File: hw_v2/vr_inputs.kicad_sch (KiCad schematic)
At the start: 26 parts, among them U1 MAX9924UAUB_, U7 74LVC2G17, U9 74LVC2G17

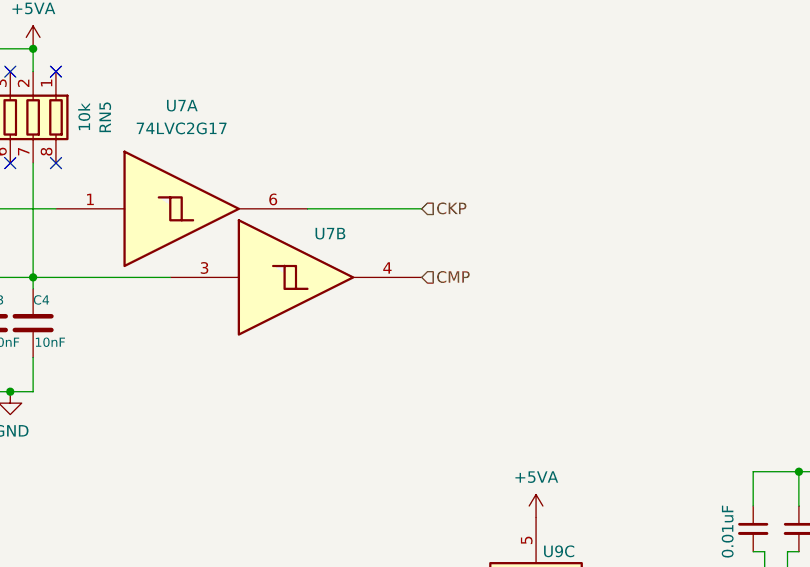
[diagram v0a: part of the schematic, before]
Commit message: hw v2
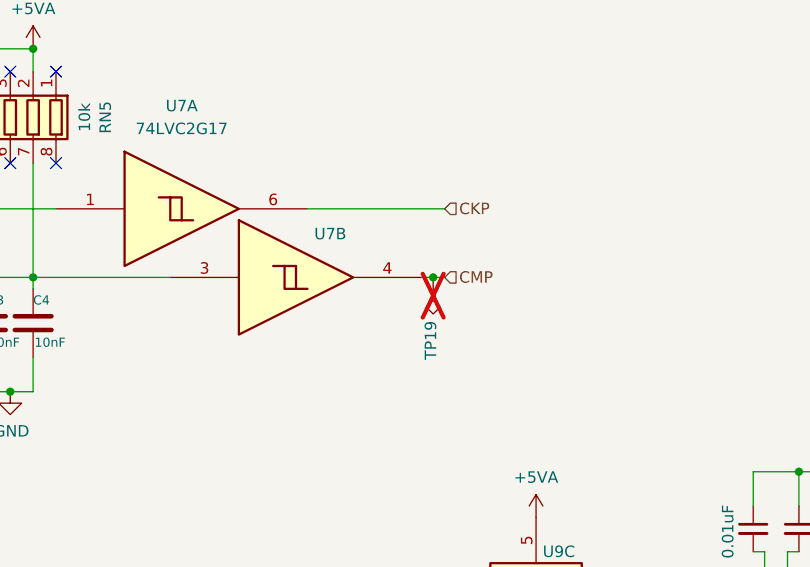
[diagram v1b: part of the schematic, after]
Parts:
- added TP19: TestPoint_Alt, TestPoint:TestPoint_Pad_1.0x1.0mm, symbol Connector:TestPoint_Alt
- U1: footprint MAX9924UAUB_:SOP50P490X110-10N -> Package_SO:MSOP-10_3x3mm_P0.5mm
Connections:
- net CMP: now also TP19.1
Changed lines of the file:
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@@
 	)
 	(junction
+		(at 123.19 135.89)
+		(diameter 0)
+		(color 0 0 0 0)
+	)
+	(junction
 		(at 54.61 43.18)
 		(diameter 0)
@@
 	(wire
 		(pts
-			(xy 121.92 128.27) (xy 109.22 128.27)
+			(xy 124.46 128.27) (xy 109.22 128.27)
+		)
+		(stroke
+			(width 0)
+			(type default)
+		)
+	)
+	(wire
+		(pts
+			(xy 124.46 135.89) (xy 123.19 135.89)
 		)
 		(stroke
@@
 	(wire
 		(pts
+			(xy 123.19 135.89) (xy 121.92 135.89)
+		)
+		(stroke
+			(width 0)
+			(type default)
+		)
+	)
+	(wire
+		(pts
 			(xy 73.66 113.03) (xy 73.66 110.49)
 		)
@@
 	(hierarchical_label "CMP"
 		(shape input)
-		(at 121.92 135.89 0)
+		(at 124.46 135.89 0)
 		(effects
 			(font
@@
 	(hierarchical_label "CKP"
 		(shape input)
-		(at 121.92 128.27 0)
+		(at 124.46 128.27 0)
 		(effects
 			(font
@@
 			)
 		)
-		(property "Footprint" "MAX9924UAUB_:SOP50P490X110-10N"
+		(property "Footprint" "Package_SO:MSOP-10_3x3mm_P0.5mm"
 			(at 133.35 69.85 0)
 			(effects
@@
 					(unit 1)
 				)
+			)
+		)
+	)
+	(symbol
+		(lib_id "Connector:TestPoint_Alt")
+		(at 123.19 135.89 180)
+		(unit 1)
+		(exclude_from_sim no)
+		(in_bom no)
+		(on_board yes)
+		(dnp yes)
+		(property "Reference" "TP19"
+			(at 122.936 140.716 90)
+			(effects
+				(font
+					(size 1.27 1.27)
+				)
+				(justify left)
+			)
+		)
+		(property "Value" "TestPoint_Alt"
+			(at 120.65 137.9221 0)
+			(effects
+				(font
+					(size 1.27 1.27)
+				)
+				(justify left)
+				(hide yes)
+			)
+		)
+		(property "Footprint" "TestPoint:TestPoint_Pad_1.0x1.0mm"
+			(at 118.11 135.89 0)
+			(effects
+				(font
+					(size 1.27 1.27)
+				)
+				(hide yes)
+			)
+		)
+		(property "Datasheet" "~"
+			(at 118.11 135.89 0)
+			(effects
+				(font
+					(size 1.27 1.27)
+				)
+				(hide yes)
+			)
+		)
+		(property "Description" "test point (alternative shape)"
+			(at 123.19 135.89 0)
+			(effects
+				(font
+					(size 1.27 1.27)
+				)
+				(hide yes)
+			)
+		)
+		(property "STOCK" "-"
+			(at 123.19 135.89 0)
+			(effects
+				(font
+					(size 1.27 1.27)
+				)
+				(hide yes)
+			)
+		)
+		(property "LCSC" "-"
+			(at 123.19 135.89 0)
+			(effects
+				(font
+					(size 1.27 1.27)
+				)
+				(hide yes)
+			)
+		)
+		(pin "1"
+		)
+		(instances
+			(project "hw_v1"
+				(path "/b3feb07e-be80-40e1-bd13-6cd54c2f8b0c/27977e95-ecc9-4124-9dfb-b7b6f545e8f2"
+					(reference "TP19")
+					(unit 1)
+				)

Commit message: fix LCSC codes
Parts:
- C1, C2, C4, C8, D13, D15, R1, R2, R4, RN5: now in the parts list
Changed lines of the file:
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@@
 		(unit 1)
 		(exclude_from_sim no)
-		(in_bom no)
+		(in_bom yes)
 		(on_board yes)
 		(dnp no)
@@
 		(unit 1)
 		(exclude_from_sim no)
-		(in_bom no)
+		(in_bom yes)
 		(on_board yes)
 		(dnp no)
@@
 		(at 163.83 163.83 0)
 		(unit 1)
-		(exclude_from_sim yes)
-		(in_bom no)
+		(exclude_from_sim no)
+		(in_bom yes)
 		(on_board yes)
 		(dnp no)
@@
 		(unit 1)
 		(exclude_from_sim no)
-		(in_bom no)
+		(in_bom yes)
 		(on_board yes)
 		(dnp no)
@@
 		(unit 1)
 		(exclude_from_sim no)
-		(in_bom no)
+		(in_bom yes)
 		(on_board yes)
 		(dnp no)
@@
 		(unit 1)
 		(exclude_from_sim no)
-		(in_bom no)
+		(in_bom yes)
 		(on_board yes)
 		(dnp no)
@@
 		(unit 1)
 		(exclude_from_sim no)
-		(in_bom no)
+		(in_bom yes)
 		(on_board yes)
 		(dnp no)
@@
 		(unit 1)
 		(exclude_from_sim no)
-		(in_bom no)
+		(in_bom yes)
 		(on_board yes)
 		(dnp no)
@@
 		(unit 1)
 		(exclude_from_sim no)
-		(in_bom no)
+		(in_bom yes)
 		(on_board yes)
 		(dnp no)
@@
 		(unit 1)
 		(exclude_from_sim no)
-		(in_bom no)
+		(in_bom yes)
 		(on_board yes)
 		(dnp no)

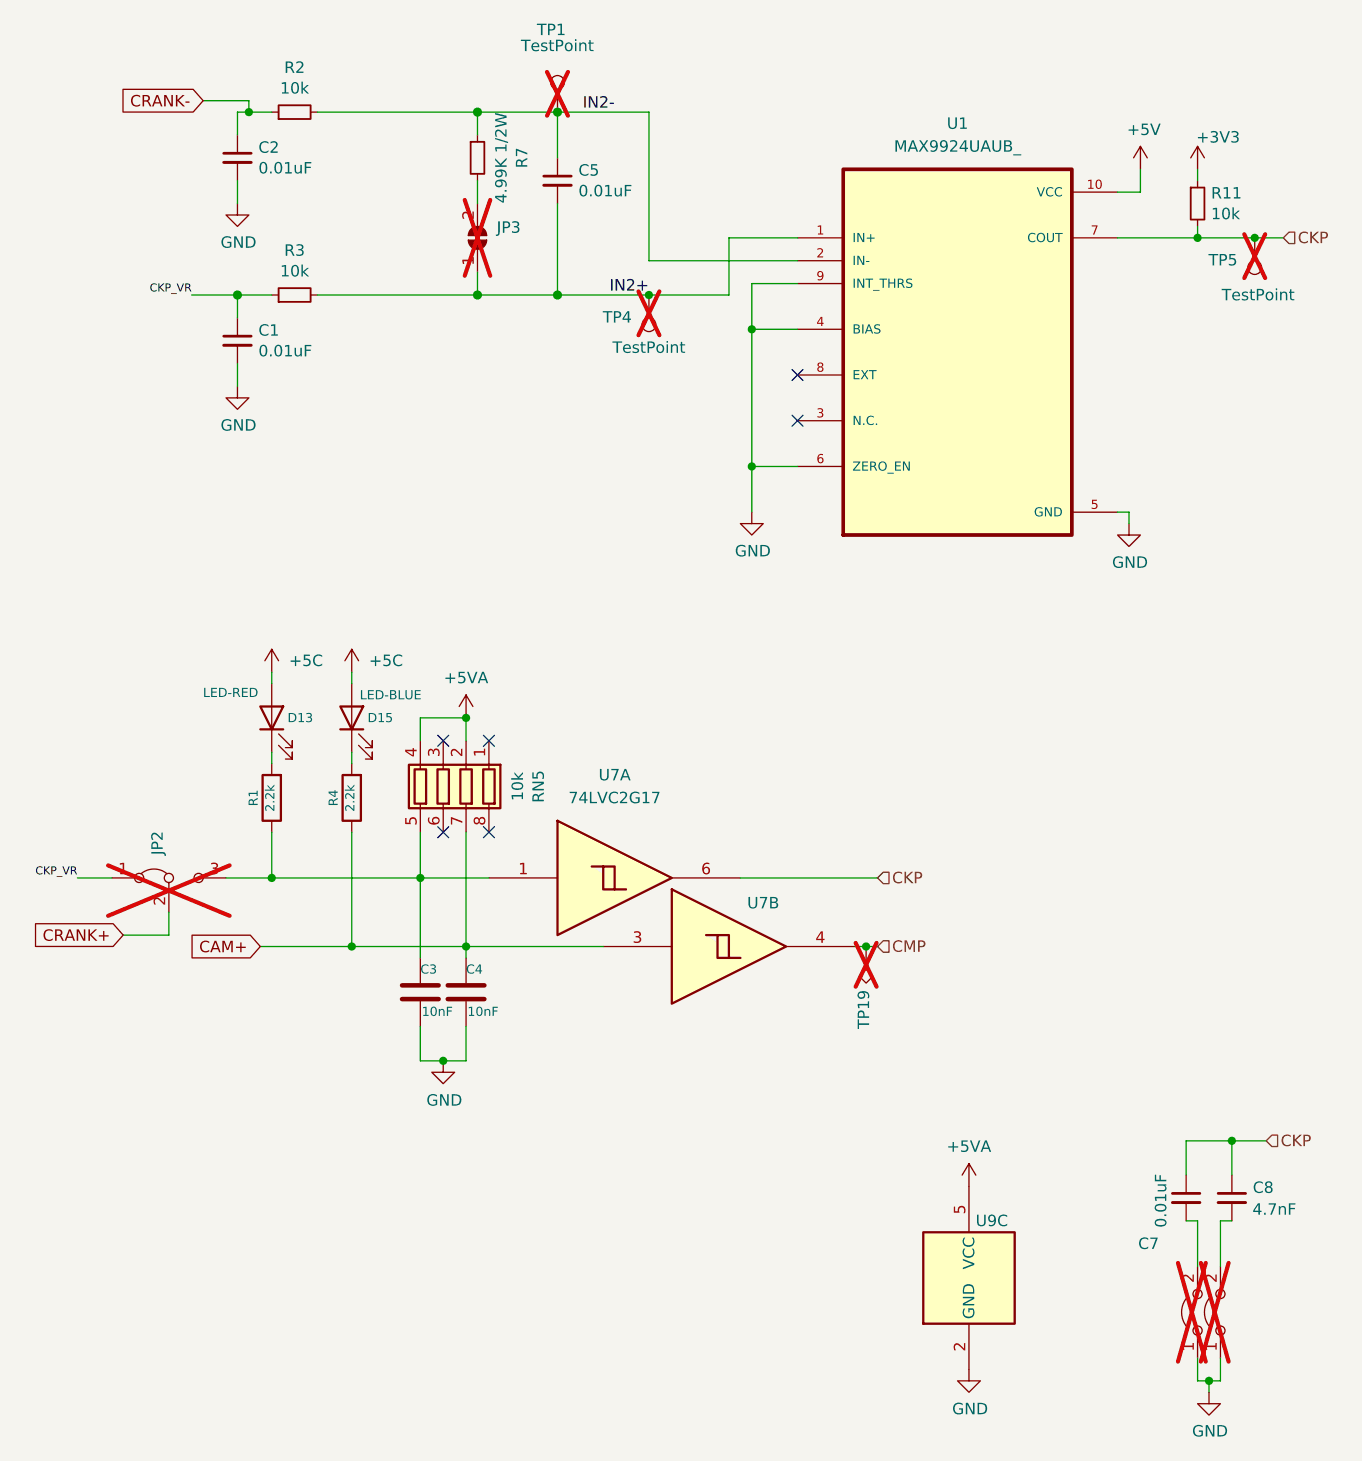
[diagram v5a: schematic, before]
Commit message: planito mas catolico
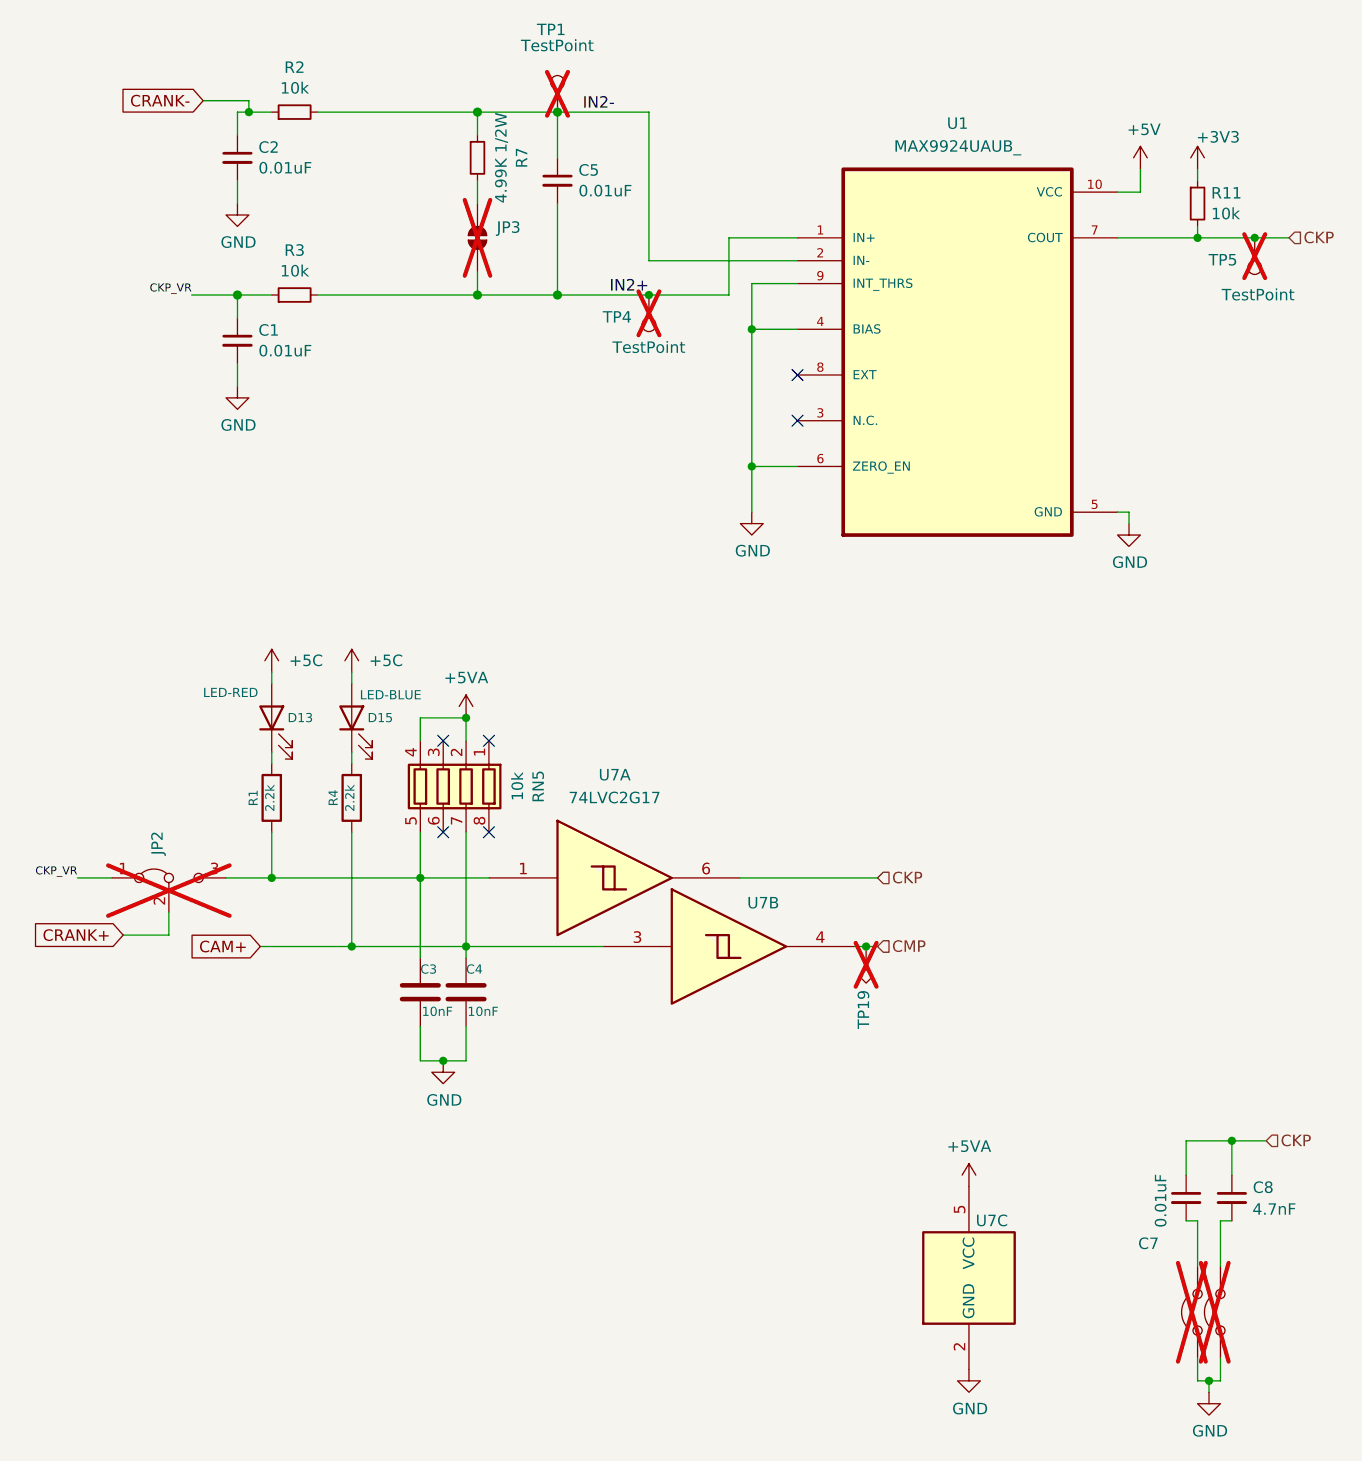
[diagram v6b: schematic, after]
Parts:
- removed U9: 74LVC2G17, Package_TO_SOT_SMD:SOT-363_SC-70-6, symbol 74xGxx:74LVC2G17
- added unit 3 of U7
- U1: footprint Package_SO:MSOP-10_3x3mm_P0.5mm -> hw_v2lib:SOP50P490X110-10N
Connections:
- net +5VA: now also U7.5 (VCC)
- net GND: now also U7.2 (GND)
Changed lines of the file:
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@@
 	(wire
 		(pts
-			(xy 166.37 57.15) (xy 169.545 57.15)
+			(xy 166.37 57.15) (xy 170.18 57.15)
 		)
 		(stroke
@@
 	(hierarchical_label "CKP"
 		(shape input)
-		(at 169.545 57.15 0)
+		(at 170.18 57.15 0)
 		(effects
 			(font
@@
 			)
 		)
-		(property "Description" ""
+		(property "Description" "Unpolarized capacitor, small symbol"
 			(at 53.34 68.58 0)
 			(effects
@@
 			)
 		)
-		(property "Datasheet" ""
+		(property "Datasheet" "~"
 			(at 78.74 140.97 0)
 			(effects
@@
 			)
 		)
-		(property "Description" ""
+		(property "Description" "Unpolarized capacitor"
 			(at 78.74 140.97 0)
 			(effects
@@
 			)
 		)
-		(property "Description" ""
+		(property "Description" "Unpolarized capacitor, small symbol"
 			(at 163.83 163.83 0)
 			(effects
@@
 	)
 	(symbol
-		(lib_id "74xGxx:74LVC2G17")
-		(at 134.62 172.72 0)
-		(unit 3)
-		(exclude_from_sim no)
-		(in_bom yes)
-		(on_board yes)
-		(dnp no)
-		(property "Reference" "U9"
-			(at 137.16 166.37 0)
-			(effects
-				(font
-					(size 1.27 1.27)
-				)
-			)
-		)
-		(property "Value" "74LVC2G17"
-			(at 133.35 163.83 0)
-			(effects
-				(font
-					(size 1.27 1.27)
-				)
-				(hide yes)
-			)
-		)
-		(property "Footprint" "Package_TO_SOT_SMD:SOT-363_SC-70-6"
-			(at 134.62 172.72 0)
-			(effects
-				(font
-					(size 1.27 1.27)
-				)
-				(hide yes)
-			)
-		)
-		(property "Datasheet" "http://www.ti.com/lit/sg/scyt129e/scyt129e.pdf"
-			(at 134.62 172.72 0)
-			(effects
-				(font
-					(size 1.27 1.27)
-				)
-				(hide yes)
-			)
-		)
-		(property "Description" "Dual Buffer, Schmitt Triggered, Low-Voltage CMOS"
-			(at 134.62 172.72 0)
-			(effects
-				(font
-					(size 1.27 1.27)
-				)
-				(hide yes)
-			)
-		)
-		(pin "3"
-		)
-		(pin "2"
-		)
-		(pin "1"
-		)
-		(pin "6"
-		)
-		(pin "4"
-		)
-		(pin "5"
-		)
-		(instances
-			(project "hw_v1"
-				(path "/b3feb07e-be80-40e1-bd13-6cd54c2f8b0c/27977e95-ecc9-4124-9dfb-b7b6f545e8f2"
-					(reference "U9")
-					(unit 3)
-				)
-			)
-		)
-	)
-	(symbol
 		(lib_id "Jumper:Jumper_3_Bridged12")
 		(at 45.72 128.27 0)
@@
 			)
 		)
-		(property "Description" ""
+		(property "Description" "Jumper, 3-pole, pins 1+2 closed/bridged"
 			(at 45.72 128.27 0)
 			(effects
@@
 			)
 		)
-		(property "Datasheet" ""
+		(property "Datasheet" "~"
 			(at 76.835 -24.765 0)
 			(effects
@@
 			)
 		)
-		(property "Description" ""
+		(property "Description" "Light emitting diode"
 			(at 57.15 110.49 0)
 			(effects
@@
 	)
 	(symbol
+		(lib_id "74xGxx:74LVC2G17")
+		(at 134.62 172.72 0)
+		(unit 3)
+		(exclude_from_sim no)
+		(in_bom yes)
+		(on_board yes)
+		(dnp no)
+		(property "Reference" "U7"
+			(at 137.16 166.37 0)
+			(effects
+				(font
+					(size 1.27 1.27)
+				)
+			)
+		)
+		(property "Value" "74LVC2G17"
+			(at 133.35 163.83 0)
+			(effects
+				(font
+					(size 1.27 1.27)
+				)
+				(hide yes)
+			)
+		)
+		(property "Footprint" "Package_TO_SOT_SMD:SOT-363_SC-70-6"
+			(at 134.62 172.72 0)
+			(effects
+				(font
+					(size 1.27 1.27)
+				)
+				(hide yes)
+			)
+		)
+		(property "Datasheet" "http://www.ti.com/lit/sg/scyt129e/scyt129e.pdf"
+			(at 134.62 172.72 0)
+			(effects
+				(font
+					(size 1.27 1.27)
+				)
+				(hide yes)
+			)
+		)
+		(property "Description" "Dual Buffer, Schmitt Triggered, Low-Voltage CMOS"
+			(at 134.62 172.72 0)
+			(effects
+				(font
+					(size 1.27 1.27)
+				)
+				(hide yes)
+			)
+		)
+		(pin "3"
+		)
+		(pin "2"
+		)
+		(pin "1"
+		)
+		(pin "6"
+		)
+		(pin "4"
+		)
+		(pin "5"
+		)
+		(instances
+			(project "hw_v1"
+				(path "/b3feb07e-be80-40e1-bd13-6cd54c2f8b0c/27977e95-ecc9-4124-9dfb-b7b6f545e8f2"
+					(reference "U7")
+					(unit 3)
+				)
+			)
+		)
+	)
+	(symbol
 		(lib_id "power:+3V3")
 		(at 160.02 49.53 0)
@@
 			)
 		)
-		(property "Description" ""
+		(property "Description" "test point"
 			(at 88.9 43.18 0)
 			(effects
@@
 			)
 		)
-		(property "Description" ""
+		(property "Description" "Unpolarized capacitor, small symbol"
 			(at 88.9 50.8 0)
 			(effects
@@
 			)
 		)
-		(property "Description" ""
+		(property "Description" "Resistor, small symbol"
 			(at 59.69 63.5 0)
 			(effects
@@
 			)
 		)
-		(property "Description" ""
+		(property "Description" "Power symbol creates a global label with name \"+5VA\""
 			(at 134.62 162.56 0)
 			(effects
@@
 			)
 		)
-		(property "Datasheet" ""
+		(property "Datasheet" "~"
 			(at 85.725 -24.765 0)
 			(effects
@@
 			)
 		)
-		(property "Description" ""
+		(property "Description" "Light emitting diode"
 			(at 66.04 110.49 0)
 			(effects
@@
 			)
 		)
-		(property "Datasheet" ""
+		(property "Datasheet" "~"
 			(at -69.215 99.695 0)
 			(effects
@@
 			)
 		)
-		(property "Description" ""
+		(property "Description" "Resistor"
 			(at 66.04 119.38 0)
 			(effects
@@
 			)
 		)
-		(property "Description" ""
+		(property "Description" "Solder Jumper, 2-pole, open"
 			(at 80.01 57.15 0)
 			(effects
@@
 			)
 		)
-		(property "Description" ""
+		(property "Description" "Unpolarized capacitor, small symbol"
 			(at 158.75 163.83 0)
 			(effects
@@
 			)
 		)
-		(property "Datasheet" ""
+		(property "Datasheet" "~"
 			(at 73.66 140.97 0)
 			(effects
@@
 			)
 		)
-		(property "Description" ""
+		(property "Description" "Unpolarized capacitor"
 			(at 73.66 140.97 0)
 			(effects
@@
 			)
 		)
-		(property "Datasheet" ""
+		(property "Datasheet" "~"
 			(at -78.105 99.695 0)
 			(effects
@@
 			)
 		)
-		(property "Description" ""
+		(property "Description" "Resistor"
 			(at 57.15 119.38 0)
 			(effects
@@
 			)
 		)
-		(property "Description" ""
+		(property "Description" "test point"
 			(at 166.37 57.15 0)
 			(effects
@@
 			)
 		)
-		(property "Description" ""
+		(property "Description" "Resistor, small symbol"
 			(at 160.02 53.34 0)
 			(effects
@@
 			)
 		)
-		(property "Description" ""
+		(property "Description" "4 resistor network, parallel topology"
 			(at 76.2 118.11 0)
 			(effects
@@
 			)
 		)
-		(property "Description" ""
+		(property "Description" "Resistor, small symbol"
 			(at 80.01 48.26 0)
 			(effects
@@
 			)
 		)
-		(property "Footprint" "Package_SO:MSOP-10_3x3mm_P0.5mm"
+		(property "Footprint" "hw_v2lib:SOP50P490X110-10N"
 			(at 133.35 69.85 0)
 			(effects
@@
 			)
 		)
-		(property "Description" ""
+		(property "Description" "test point"
 			(at 99.06 63.5 0)
 			(effects
@@
 			)
 		)
-		(property "Description" ""
+		(property "Description" "Resistor, small symbol"
 			(at 59.69 43.18 0)
 			(effects
@@
 			)
 		)
-		(property "Description" ""
+		(property "Description" "Unpolarized capacitor, small symbol"
 			(at 53.34 48.26 0)
 			(effects
@@
 			)
 		)
-		(property "Description" ""
+		(property "Description" "Power symbol creates a global label with name \"+5VA\""
 			(at 78.74 110.49 0)
 			(effects
